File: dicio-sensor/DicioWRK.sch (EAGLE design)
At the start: 59 parts, among them J1 WTB-2, J2 WTB-2, J6 WTB-2, J7 TERM10, Q1 BSS84, Q2 BSS84, Q3 BSS84, Q4 BSS84, Q5 BSS84, U1 78MM6610+PSU, U2 TSL250RD, U3 MCP9700, U4 DK-1A-L2-3, U5 RAC01-3.3, U9 MCP3202SOIC

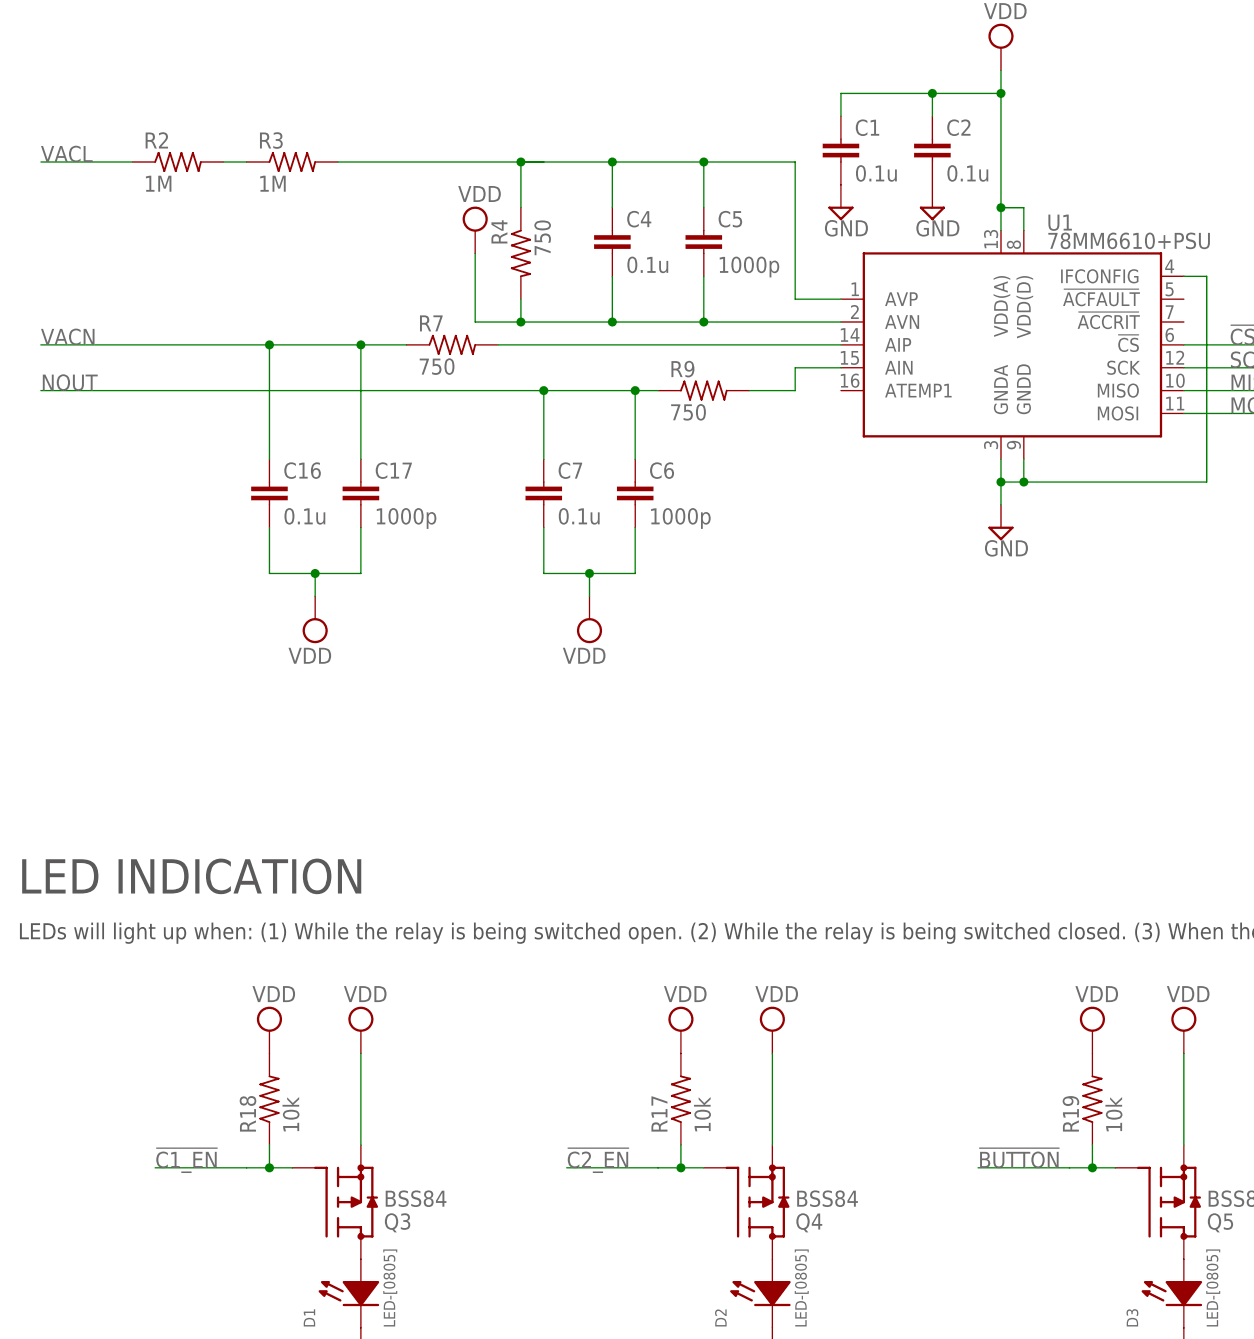
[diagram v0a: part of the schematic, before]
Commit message: R1-Out for Fab.
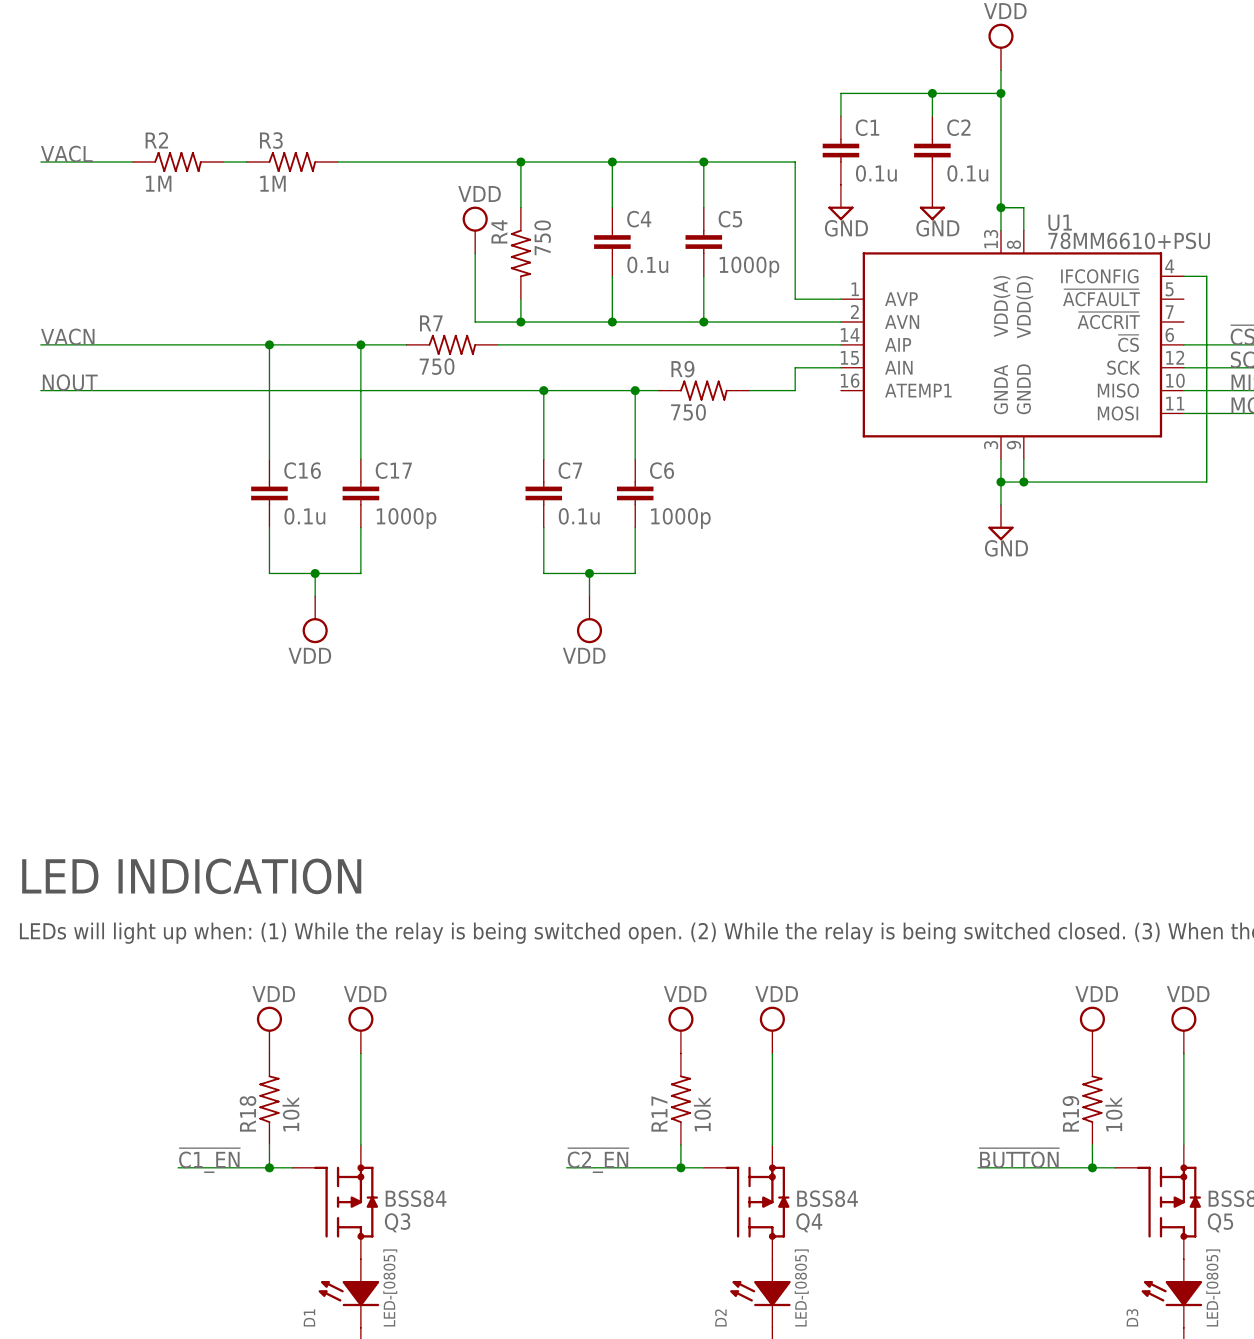
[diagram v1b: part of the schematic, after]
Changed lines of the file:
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@@
 <net name="!C1_EN!" class="0">
-<segment>
-<wire x1="40.64" y1="50.8" x2="30.48" y2="50.8" width="0.1524" layer="91"/>
-<label x="30.48" y="50.8" size="1.778" layer="95"/>
-</segment>
 <segment>
 <pinref part="R14" gate="G$1" pin="1"/>
@@
 <wire x1="45.72" y1="50.8" x2="43.18" y2="50.8" width="0.1524" layer="91"/>
 <pinref part="R18" gate="G$1" pin="1"/>
-<wire x1="43.18" y1="50.8" x2="40.64" y2="50.8" width="0.1524" layer="91"/>
+<wire x1="43.18" y1="50.8" x2="33.02" y2="50.8" width="0.1524" layer="91"/>
 <wire x1="43.18" y1="50.8" x2="43.18" y2="53.34" width="0.1524" layer="91"/>
 <junction x="43.18" y="50.8"/>
+<label x="33.02" y="50.8" size="1.778" layer="95"/>
 </segment>
 <segment>
@@
 </net>
 <net name="!C2_EN!" class="0">
-<segment>
-<wire x1="86.36" y1="50.8" x2="76.2" y2="50.8" width="0.1524" layer="91"/>
-<label x="76.2" y="50.8" size="1.778" layer="95"/>
-</segment>
 <segment>
 <pinref part="R13" gate="G$1" pin="1"/>
@@
 <pinref part="R17" gate="G$1" pin="1"/>
 <wire x1="88.9" y1="53.34" x2="88.9" y2="50.8" width="0.1524" layer="91"/>
-<wire x1="88.9" y1="50.8" x2="86.36" y2="50.8" width="0.1524" layer="91"/>
+<wire x1="88.9" y1="50.8" x2="76.2" y2="50.8" width="0.1524" layer="91"/>
 <pinref part="Q4" gate="G$1" pin="G"/>
 <wire x1="91.44" y1="50.8" x2="88.9" y2="50.8" width="0.1524" layer="91"/>
 <junction x="88.9" y="50.8"/>
+<label x="76.2" y="50.8" size="1.778" layer="95"/>
 </segment>
 <segment>
@@
 <net name="!BUTTON!" class="0">
 <segment>
-<wire x1="132.08" y1="50.8" x2="121.92" y2="50.8" width="0.1524" layer="91"/>
-<label x="121.92" y="50.8" size="1.778" layer="95"/>
-</segment>
-<segment>
 <pinref part="R22" gate="G$1" pin="2"/>
 <pinref part="C13" gate="G$1" pin="1"/>
@@
 <wire x1="137.16" y1="50.8" x2="134.62" y2="50.8" width="0.1524" layer="91"/>
 <wire x1="134.62" y1="50.8" x2="134.62" y2="53.34" width="0.1524" layer="91"/>
-<wire x1="134.62" y1="50.8" x2="132.08" y2="50.8" width="0.1524" layer="91"/>
+<wire x1="134.62" y1="50.8" x2="121.92" y2="50.8" width="0.1524" layer="91"/>
 <junction x="134.62" y="50.8"/>
+<label x="121.92" y="50.8" size="1.778" layer="95"/>
 </segment>
 </net>
 <net name="N$1" class="0">
 <segment>
-<pinref part="R4" gate="G$1" pin="1"/>
-<wire x1="71.12" y1="157.48" x2="71.12" y2="162.56" width="0.1524" layer="91"/>
-<pinref part="R3" gate="G$1" pin="2"/>
-<wire x1="71.12" y1="162.56" x2="50.8" y2="162.56" width="0.1524" layer="91"/>
 <pinref part="U1" gate="G$1" pin="AVP"/>
-<wire x1="71.12" y1="162.56" x2="81.28" y2="162.56" width="0.1524" layer="91"/>
-<junction x="71.12" y="162.56"/>
 <wire x1="81.28" y1="162.56" x2="91.44" y2="162.56" width="0.1524" layer="91"/>
 <wire x1="91.44" y1="162.56" x2="101.6" y2="162.56" width="0.1524" layer="91"/>
@@
 <pinref part="C4" gate="G$1" pin="1"/>
 <wire x1="81.28" y1="157.48" x2="81.28" y2="162.56" width="0.1524" layer="91"/>
+<pinref part="R4" gate="G$1" pin="1"/>
+<wire x1="71.12" y1="157.48" x2="71.12" y2="162.56" width="0.1524" layer="91"/>
+<wire x1="71.12" y1="162.56" x2="81.28" y2="162.56" width="0.1524" layer="91"/>
 <junction x="81.28" y="162.56"/>
+<pinref part="R3" gate="G$1" pin="2"/>
+<wire x1="71.12" y1="162.56" x2="50.8" y2="162.56" width="0.1524" layer="91"/>
+<junction x="71.12" y="162.56"/>
 </segment>
 </net>
@@
 </segment>
 </net>
-<net name="N$9" class="0">
-<segment>
-<wire x1="71.12" y1="162.56" x2="73.66" y2="162.56" width="0.1524" layer="91"/>
-</segment>
-</net>
